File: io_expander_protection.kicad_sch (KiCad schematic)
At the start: 72 parts

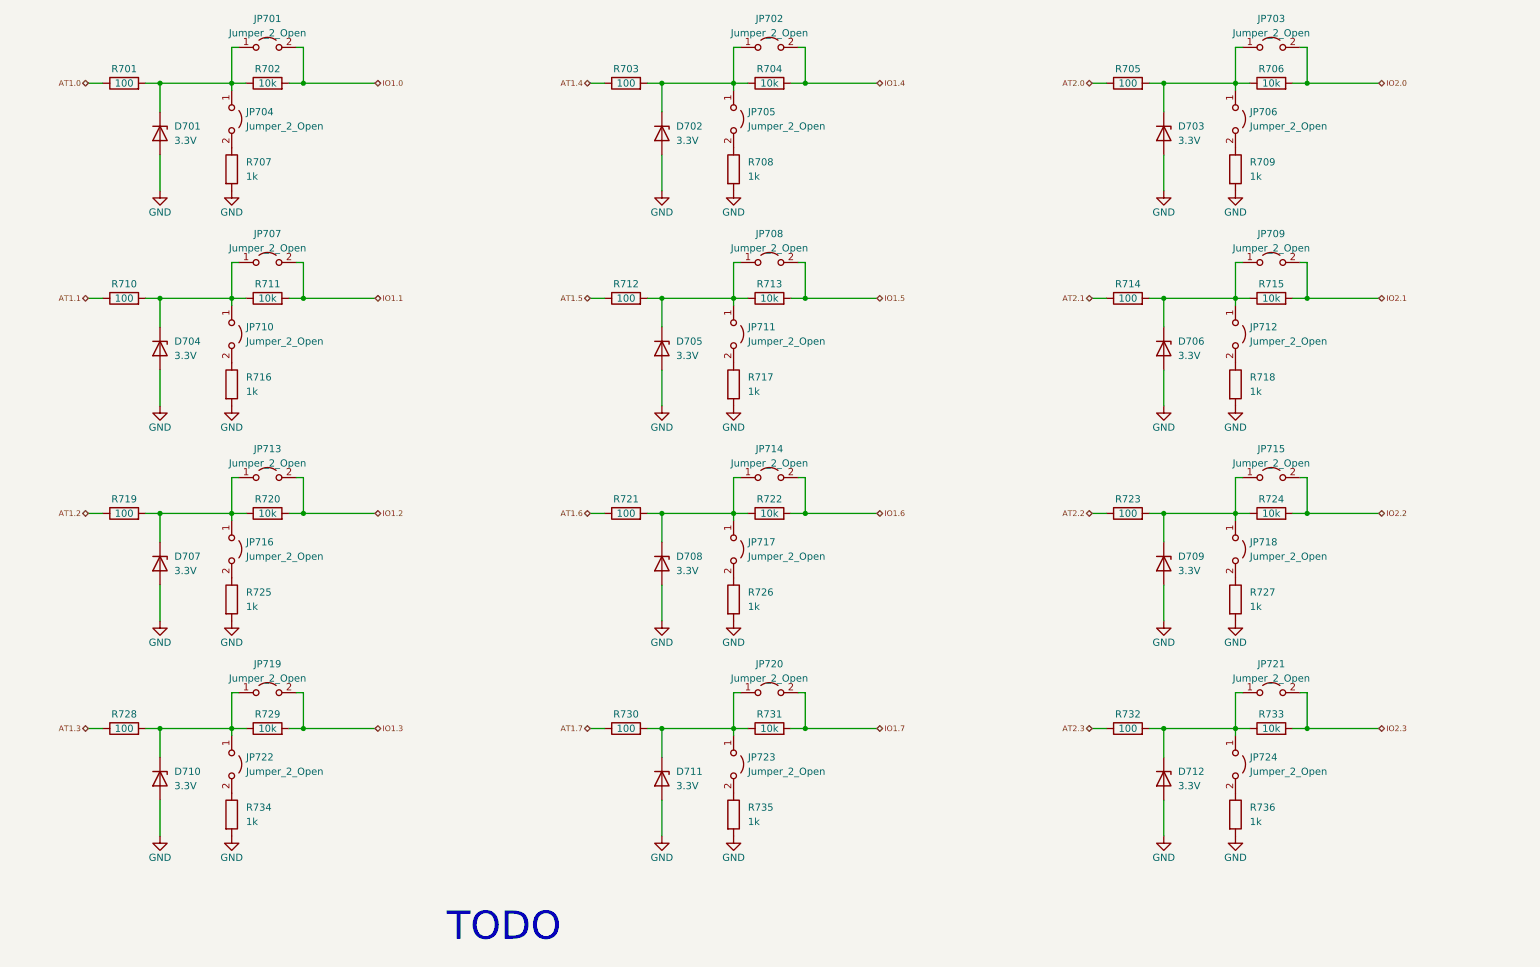
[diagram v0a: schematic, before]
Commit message: started routing
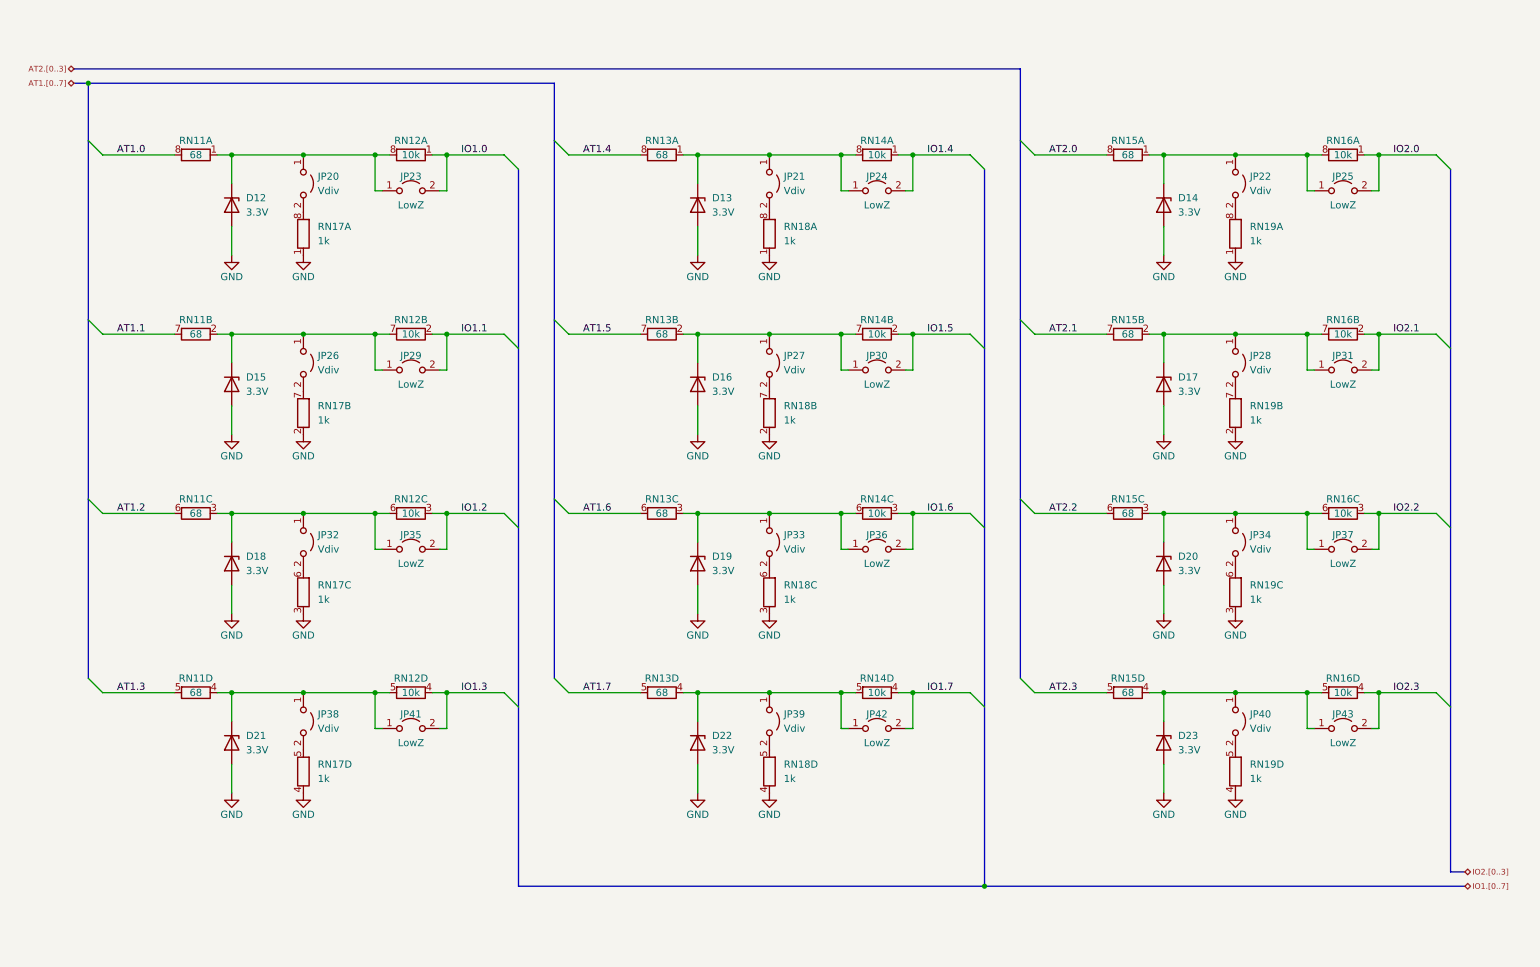
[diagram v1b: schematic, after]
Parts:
- removed D701, D702, D703, D704, D705, D706, D707, D708, D709, D710, D711, D712: 3.3V, symbol Device:D_Zener
- removed JP701, JP702, JP703, JP704, JP705, JP706, JP707, JP708, JP709, JP710, JP711, JP712, JP713, JP714, JP715, JP716, JP717, JP718, JP719, JP720, JP721, JP722, JP723, JP724: Jumper_2_Open, symbol Jumper:Jumper_2_Open
- removed R701, R703, R705, R710, R712, R714, R719, R721, R723, R728, R730, R732: 100, symbol Device:R
- removed R702, R704, R706, R711, R713, R715, R720, R722, R724, R729, R731, R733: 10k, symbol Device:R
- removed R707, R708, R709, R716, R717, R718, R725, R726, R727, R734, R735, R736: 1k, symbol Device:R
- added D12, D13, D14, D15, D16, D17, D18, D19, D20, D21, D22, D23: 3.3V, Diode_SMD:D_SOD-123, symbol Device:D_Zener
- added JP20, JP21, JP22, JP26, JP27, JP28, JP32, JP33, JP34, JP38, JP39, JP40: Vdiv, Jumper:SolderJumper-2_P1.3mm_Open_TrianglePad1.0x1.5mm, symbol Jumper:Jumper_2_Open
- added JP23, JP24, JP25, JP29, JP30, JP31, JP35, JP36, JP37, JP41, JP42, JP43: LowZ, Jumper:SolderJumper-2_P1.3mm_Open_TrianglePad1.0x1.5mm, symbol Jumper:Jumper_2_Open
- added RN11, RN13, RN15: 68, Resistor_SMD:R_Array_Convex_4x0603, symbol Device:R_Pack04_Split
- added RN12, RN14, RN16: 10k, Resistor_SMD:R_Array_Convex_4x0603, symbol Device:R_Pack04_Split
- added RN17, RN18, RN19: 1k, Resistor_SMD:R_Array_Convex_4x0603, symbol Device:R_Pack04_Split
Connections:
- net AT1.0: now also RN11.8 (R1.2)
- net AT1.1: now also RN11.7 (R2.2)
- net AT1.2: now also RN11.6 (R3.2)
- net AT1.3: now also RN11.5 (R4.2)
- net AT1.4: now also RN13.8 (R1.2)
- net AT1.5: now also RN13.7 (R2.2)
- net AT1.6: now also RN13.6 (R3.2)
- net AT1.7: now also RN13.5 (R4.2)
- net AT2.0: now also RN15.8 (R1.2)
- net AT2.1: now also RN15.7 (R2.2)
- net AT2.2: now also RN15.6 (R3.2)
- net AT2.3: now also RN15.5 (R4.2)
- net GND: now also D12.2 (A), D13.2 (A), D14.2 (A), D15.2 (A), D16.2 (A), D17.2 (A), D18.2 (A), D19.2 (A), D20.2 (A), D21.2 (A), D22.2 (A), D23.2 (A), RN17.1 (R1.1), RN17.2 (R2.1), RN17.3 (R3.1), RN17.4 (R4.1), RN18.1 (R1.1), RN18.2 (R2.1), RN18.3 (R3.1), RN18.4 (R4.1), RN19.1 (R1.1), RN19.2 (R2.1), RN19.3 (R3.1), RN19.4 (R4.1)
- net IO1.0: now also JP23.2 (B), RN12.1 (R1.1)
- net IO1.1: now also JP29.2 (B), RN12.2 (R2.1)
- net IO1.2: now also JP35.2 (B), RN12.3 (R3.1)
- net IO1.3: now also JP41.2 (B), RN12.4 (R4.1)
- net IO1.4: now also JP24.2 (B), RN14.1 (R1.1)
- net IO1.5: now also JP30.2 (B), RN14.2 (R2.1)
- net IO1.6: now also JP36.2 (B), RN14.3 (R3.1)
- net IO1.7: now also JP42.2 (B), RN14.4 (R4.1)
- net IO2.0: now also JP25.2 (B), RN16.1 (R1.1)
- net IO2.1: now also JP31.2 (B), RN16.2 (R2.1)
- net IO2.2: now also JP37.2 (B), RN16.3 (R3.1)
- net IO2.3: now also JP43.2 (B), RN16.4 (R4.1)
- new net: D17.1 (K), JP28.1 (A), JP31.1 (A), RN15.2 (R2.1), RN16.7 (R2.2)
- new net: JP28.2 (B), RN19.7 (R2.2)
- new net: D22.1 (K), JP39.1 (A), JP42.1 (A), RN13.4 (R4.1), RN14.5 (R4.2)
- new net: D19.1 (K), JP33.1 (A), JP36.1 (A), RN13.3 (R3.1), RN14.6 (R3.2)
- new net: JP32.2 (B), RN17.6 (R3.2)
- new net: D20.1 (K), JP34.1 (A), JP37.1 (A), RN15.3 (R3.1), RN16.6 (R3.2)
- new net: D12.1 (K), JP20.1 (A), JP23.1 (A), RN11.1 (R1.1), RN12.8 (R1.2)
- new net: D13.1 (K), JP21.1 (A), JP24.1 (A), RN13.1 (R1.1), RN14.8 (R1.2)
- new net: JP21.2 (B), RN18.8 (R1.2)
- new net: JP26.2 (B), RN17.7 (R2.2)
- new net: D14.1 (K), JP22.1 (A), JP25.1 (A), RN15.1 (R1.1), RN16.8 (R1.2)
- new net: D15.1 (K), JP26.1 (A), JP29.1 (A), RN11.2 (R2.1), RN12.7 (R2.2)
- new net: JP33.2 (B), RN18.6 (R3.2)
- new net: D21.1 (K), JP38.1 (A), JP41.1 (A), RN11.4 (R4.1), RN12.5 (R4.2)
- new net: JP38.2 (B), RN17.5 (R4.2)
- new net: D23.1 (K), JP40.1 (A), JP43.1 (A), RN15.4 (R4.1), RN16.5 (R4.2)
- new net: D18.1 (K), JP32.1 (A), JP35.1 (A), RN11.3 (R3.1), RN12.6 (R3.2)
- new net: D16.1 (K), JP27.1 (A), JP30.1 (A), RN13.2 (R2.1), RN14.7 (R2.2)
- new net: JP39.2 (B), RN18.5 (R4.2)
- new net: JP34.2 (B), RN19.6 (R3.2)
- new net: JP20.2 (B), RN17.8 (R1.2)
- new net: JP22.2 (B), RN19.8 (R1.2)
- new net: JP40.2 (B), RN19.5 (R4.2)
- new net: JP27.2 (B), RN18.7 (R2.2)
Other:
- note removed: "TODO"
- title: (none) -> [canbrd] CAN/RS485 IO board

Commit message: Done?
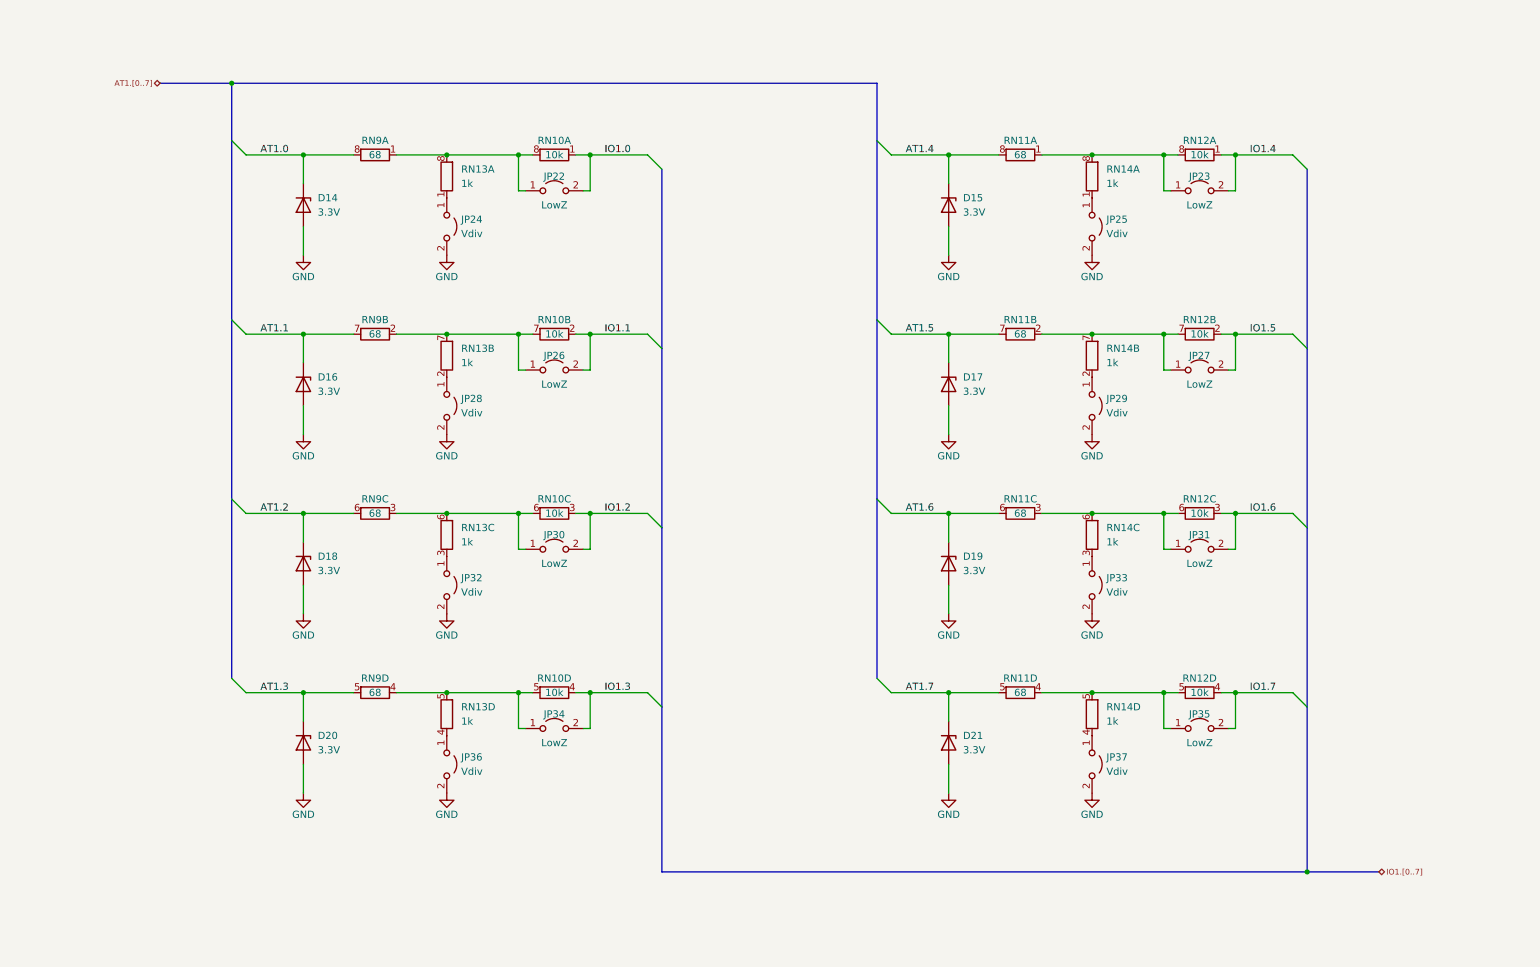
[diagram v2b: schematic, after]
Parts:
- removed D12, D13, D22, D23: 3.3V, Diode_SMD:D_SOD-123, symbol Device:D_Zener
- removed JP20, JP21, JP38, JP39, JP40: Vdiv, Jumper:SolderJumper-2_P1.3mm_Open_TrianglePad1.0x1.5mm, symbol Jumper:Jumper_2_Open
- removed JP41, JP42, JP43: LowZ, Jumper:SolderJumper-2_P1.3mm_Open_TrianglePad1.0x1.5mm, symbol Jumper:Jumper_2_Open
- removed RN15: 68, Resistor_SMD:R_Array_Convex_4x0603, symbol Device:R_Pack04_Split
- removed RN16: 10k, Resistor_SMD:R_Array_Convex_4x0603, symbol Device:R_Pack04_Split
- removed RN17, RN18, RN19: 1k, Resistor_SMD:R_Array_Convex_4x0603, symbol Device:R_Pack04_Split
- added RN10: 10k, Resistor_SMD:R_Array_Convex_4x0603, symbol Device:R_Pack04_Split
- added RN9: 68, Resistor_SMD:R_Array_Convex_4x0603, symbol Device:R_Pack04_Split
- JP22, JP26, JP27, JP34: value Vdiv -> LowZ
- JP24, JP25, JP29, JP36, JP37: value LowZ -> Vdiv
- RN13: value 68 -> 1k
- RN14: value 10k -> 1k
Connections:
- net IO2.0 is gone; now on net GND: JP25.2 (B)
- net IO2.1 is gone; now on net IO1.6: JP31.2 (B)
- net IO2.2 is gone; now on net GND: JP37.2 (B)
- net AT1.0: now also D14.1 (K), RN9.8 (R1.2); no longer RN11.8 (R1.2)
- net AT1.1: now also D16.1 (K), RN9.7 (R2.2); no longer RN11.7 (R2.2)
- net AT1.2: now also D18.1 (K), RN9.6 (R3.2); no longer RN11.6 (R3.2)
- net AT1.3: now also D20.1 (K), RN9.5 (R4.2); no longer RN11.5 (R4.2)
- net AT1.4: now also D15.1 (K), RN11.8 (R1.2); no longer RN13.8 (R1.2)
- net AT1.5: now also D17.1 (K), RN11.7 (R2.2); no longer RN13.7 (R2.2)
- net AT1.6: now also D19.1 (K), RN11.6 (R3.2); no longer RN13.6 (R3.2)
- net AT1.7: now also D21.1 (K), RN11.5 (R4.2); no longer RN13.5 (R4.2)
- net GND: now also JP24.2 (B), JP28.2 (B), JP29.2 (B), JP32.2 (B), JP33.2 (B), JP36.2 (B)
- net IO1.0: now also JP22.2 (B), RN10.1 (R1.1); no longer JP23.2 (B), RN12.1 (R1.1)
- net IO1.1: now also JP26.2 (B), RN10.2 (R2.1); no longer JP29.2 (B), RN12.2 (R2.1)
- net IO1.2: now also JP30.2 (B), RN10.3 (R3.1); no longer JP35.2 (B), RN12.3 (R3.1)
- net IO1.3: now also JP34.2 (B), RN10.4 (R4.1); no longer RN12.4 (R4.1)
- net IO1.4: now also JP23.2 (B), RN12.1 (R1.1); no longer JP24.2 (B), RN14.1 (R1.1)
- net IO1.5: now also JP27.2 (B), RN12.2 (R2.1); no longer JP30.2 (B), RN14.2 (R2.1)
- net IO1.6: now also RN12.3 (R3.1); no longer JP36.2 (B), RN14.3 (R3.1)
- net IO1.7: now also JP35.2 (B), RN12.4 (R4.1); no longer RN14.4 (R4.1)
- net at RN13.4 (R4.1): now also JP36.1 (A); no longer RN14.5 (R4.2)
- net at JP23.1 (A), RN11.1 (R1.1), RN12.8 (R1.2): now also RN14.8 (R1.2)
- net at JP24.1 (A), RN13.1 (R1.1): no longer RN14.8 (R1.2)
- net at RN11.4 (R4.1), RN12.5 (R4.2): now also JP35.1 (A), RN14.5 (R4.2); no longer D21.1 (K)
- new net: JP25.1 (A), RN14.1 (R1.1)
- new net: JP27.1 (A), RN11.2 (R2.1), RN12.7 (R2.2), RN14.7 (R2.2)
- new net: JP32.1 (A), RN13.3 (R3.1)
- new net: JP26.1 (A), RN10.7 (R2.2), RN13.7 (R2.2), RN9.2 (R2.1)
- new net: JP30.1 (A), RN10.6 (R3.2), RN13.6 (R3.2), RN9.3 (R3.1)
- new net: JP34.1 (A), RN10.5 (R4.2), RN13.5 (R4.2), RN9.4 (R4.1)
- new net: JP28.1 (A), RN13.2 (R2.1)
- new net: JP29.1 (A), RN14.2 (R2.1)
- new net: JP33.1 (A), RN14.3 (R3.1)
- new net: JP22.1 (A), RN10.8 (R1.2), RN13.8 (R1.2), RN9.1 (R1.1)
- new net: JP31.1 (A), RN11.3 (R3.1), RN12.6 (R3.2), RN14.6 (R3.2)
- new net: JP37.1 (A), RN14.4 (R4.1)
